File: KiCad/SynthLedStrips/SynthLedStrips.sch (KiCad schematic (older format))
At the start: 38 parts, among them J1 XLR4, J2 XLR4, J3 MIDI IN Kronos DIN-5, J4 MIDI OUT Kronos DIN-5, J5 MIDI IN Acuna DIN-5, J6 MIDI OUT Acuna DIN-5, J7 Conn_01x02_Female, U1 ESP32-WROOM-32, U2 74HC14, U3 74HC14, U4 6N138, U6 6N138

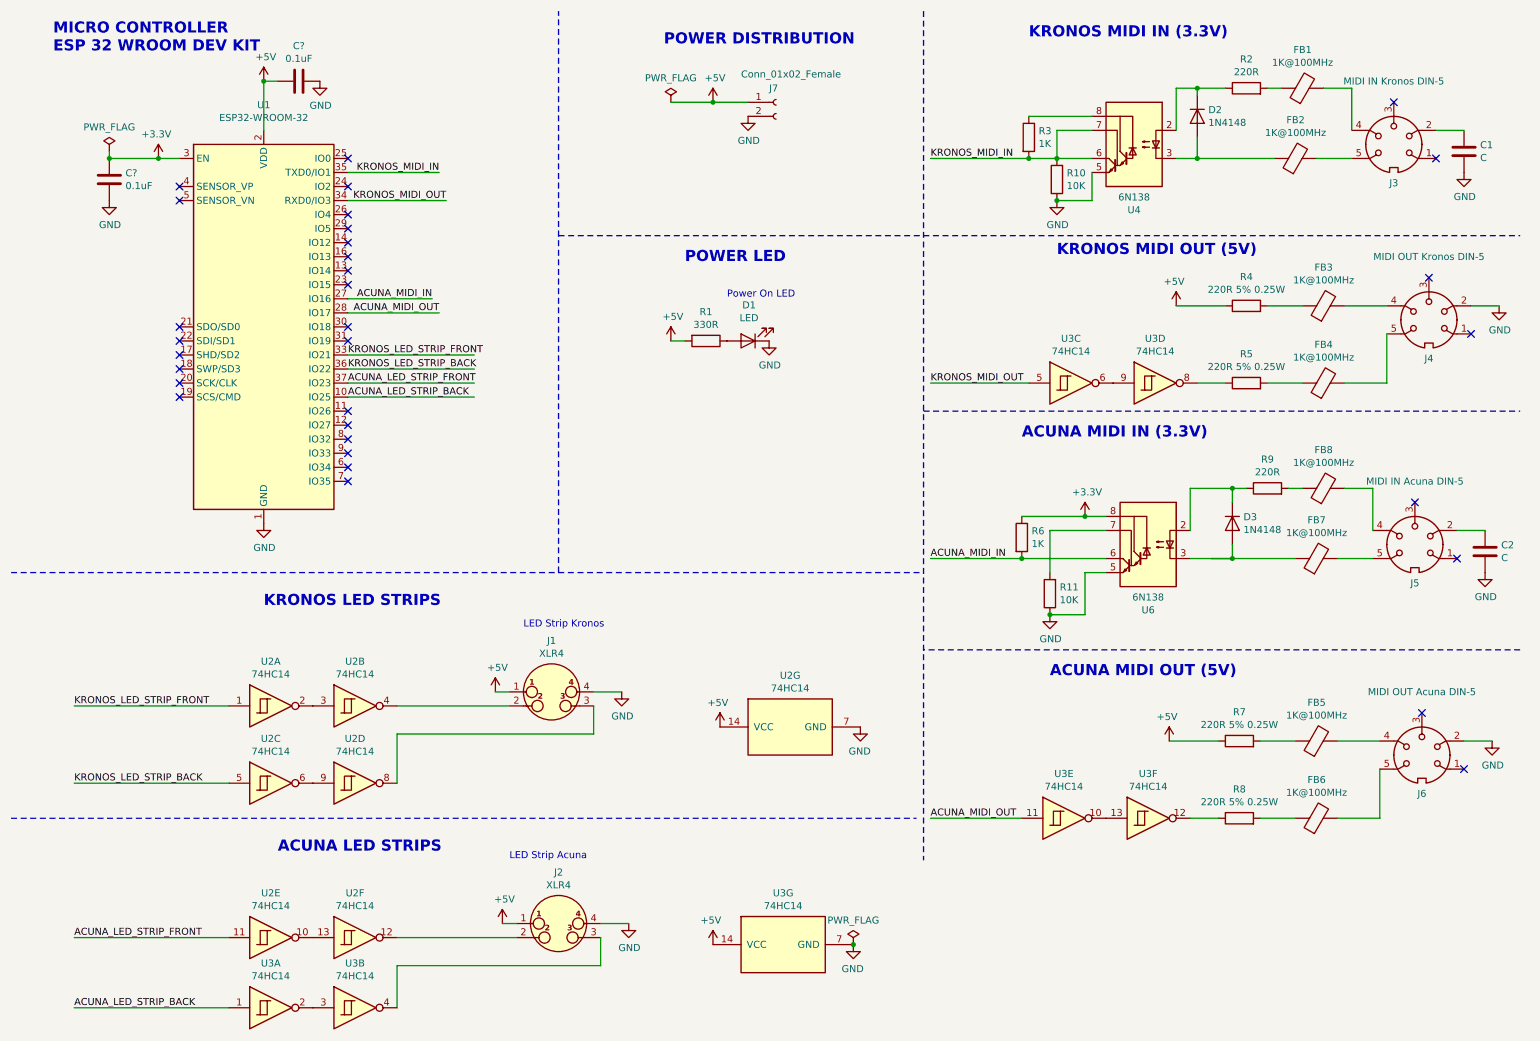
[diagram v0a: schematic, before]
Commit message: KiCad project
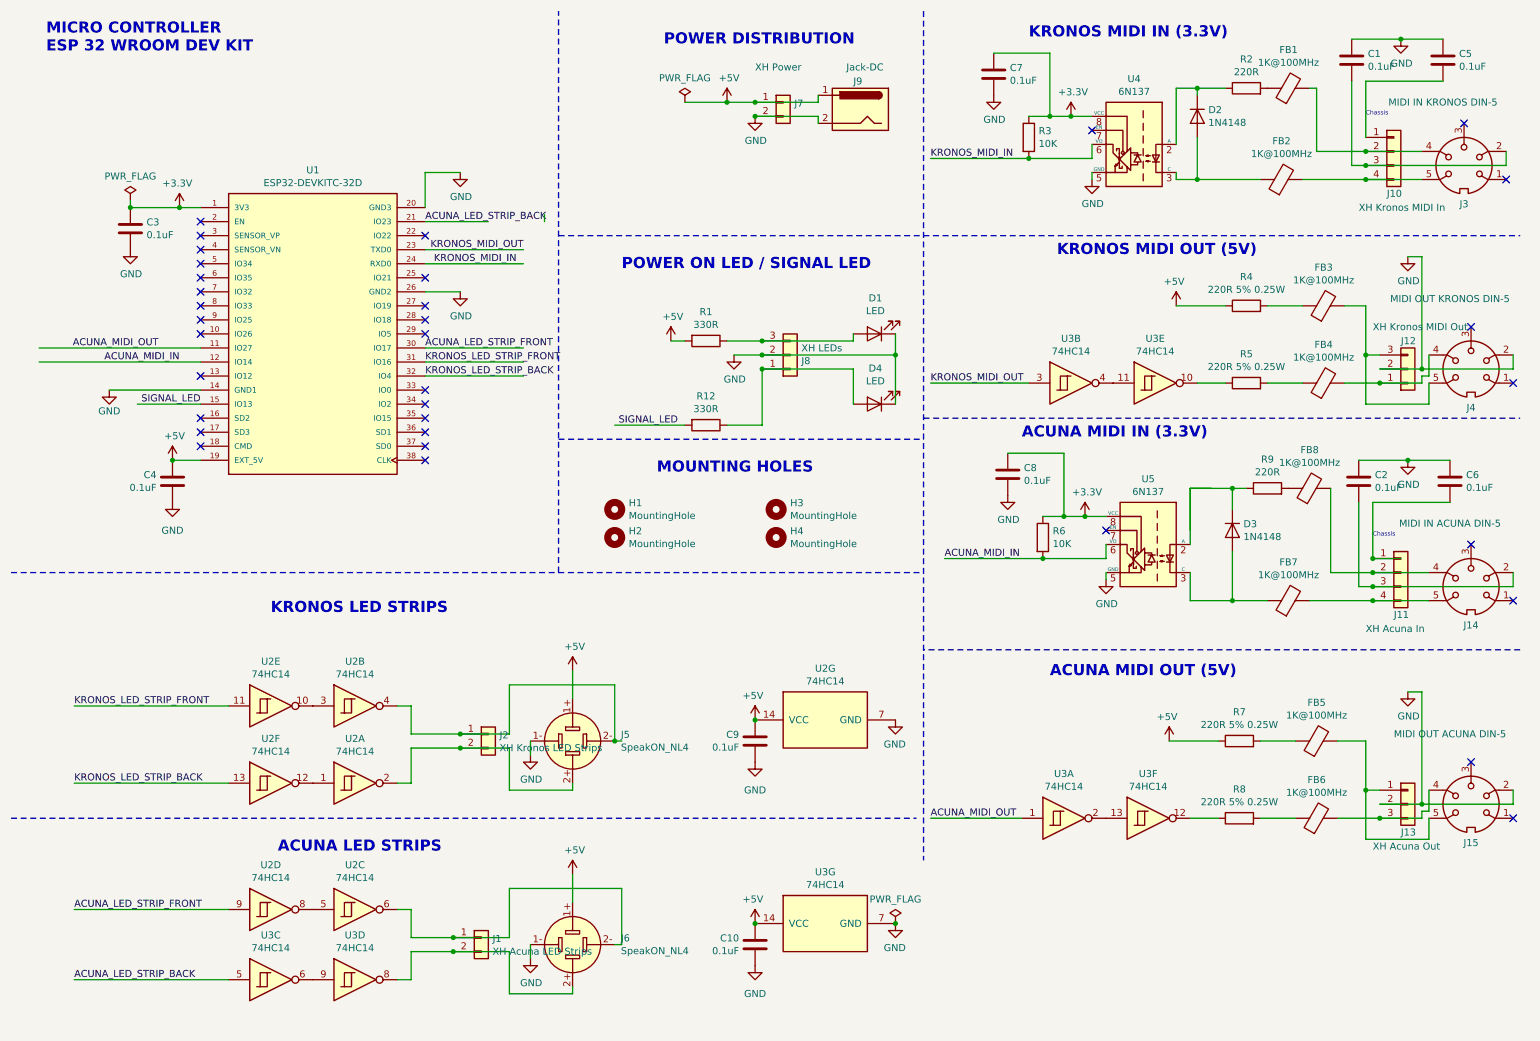
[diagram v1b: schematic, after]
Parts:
- removed J1, J2: XLR4, symbol Connector:XLR4
- removed J5: MIDI IN Acuna DIN-5, symbol Connector:DIN-5
- removed J6: MIDI OUT Acuna DIN-5, symbol Connector:DIN-5
- removed J7: Conn_01x02_Female, symbol Connector:Conn_01x02_Female
- removed R10, R11: 10K, symbol Device:R
- removed U1: ESP32-WROOM-32, RF_Module:ESP32-WROOM-32, symbol RF_Module:ESP32-WROOM-32
- removed U4, U6: 6N138, symbol Isolator:6N138
- added C10, C5, C6, C7, C8, C9: 0.1uF, Capacitor_SMD:C_0805_2012Metric_Pad1.15x1.40mm_HandSolder, symbol Device:C
- added D4: LED, symbol Device:LED
- added H1, H2, H3, H4: MountingHole, MountingHole:MountingHole_4.3mm_M4, symbol Mechanical:MountingHole
- added J1: XH Acuna LED Strips, Connector_JST:JST_XH_B2B-XH-A_1x02_P2.50mm_Vertical, symbol Connector_Generic:Conn_01x02
- added J10: XH Kronos MIDI In, Connector_JST:JST_XH_B4B-XH-A_1x04_P2.50mm_Vertical, symbol Connector_Generic:Conn_01x04
- added J11: XH Acuna In, Connector_JST:JST_XH_B4B-XH-A_1x04_P2.50mm_Vertical, symbol Connector_Generic:Conn_01x04
- added J12: XH Kronos MIDI Out, Connector_JST:JST_XH_B3B-XH-A_1x03_P2.50mm_Vertical, symbol Connector_Generic:Conn_01x03
- added J13: XH Acuna Out, Connector_JST:JST_XH_B3B-XH-A_1x03_P2.50mm_Vertical, symbol Connector_Generic:Conn_01x03
- added J14: MIDI IN ACUNA DIN-5, symbol Connector:DIN-5
- added J15: MIDI OUT ACUNA DIN-5, symbol Connector:DIN-5
- added J2: XH Kronos LED Strips, Connector_JST:JST_XH_B2B-XH-A_1x02_P2.50mm_Vertical, symbol Connector_Generic:Conn_01x02
- added J5, J6: SpeakON_NL4, symbol Connector:SpeakON_NL4
- added J7: XH Power, Connector_JST:JST_XH_B2B-XH-A_1x02_P2.50mm_Vertical, symbol Connector_Generic:Conn_01x02
- added J8: XH LEDs, Connector_JST:JST_XH_B3B-XH-A_1x03_P2.50mm_Vertical, symbol Connector_Generic:Conn_01x03
- added J9: Jack-DC, symbol Connector:Jack-DC
- added R12: 330R, Resistor_SMD:R_0805_2012Metric_Pad1.15x1.40mm_HandSolder, symbol Device:R
- added U1: ESP32-DEVKITC-32D, ESP32_DevKit:MODULE_ESP32-DEVKITC-32D, symbol ESP32_DevKit:ESP32-DEVKITC-32D
- added U4, U5: 6N137, 6N137S:8-SMD, symbol Isolator:6N137
- C1, C2: value C -> 0.1uF; footprint (none) -> Capacitor_SMD:C_0805_2012Metric_Pad1.15x1.40mm_HandSolder
- C3, C4: renamed from C?; footprint (none) -> Capacitor_SMD:C_0805_2012Metric_Pad1.15x1.40mm_HandSolder
- D2, D3: footprint (none) -> Diode_SMD:D_SOD-323_HandSoldering
- FB1, FB2, FB3, FB4, FB5, FB6, FB7, FB8: footprint (none) -> Fuse:Fuse_1210_3225Metric_Pad1.42x2.65mm_HandSolder
- J3: value MIDI IN Kronos DIN-5 -> MIDI IN KRONOS DIN-5
- J4: value MIDI OUT Kronos DIN-5 -> MIDI OUT KRONOS DIN-5
- R1, R2, R9: footprint (none) -> Resistor_SMD:R_0805_2012Metric_Pad1.15x1.40mm_HandSolder
- R3, R6: value 1K -> 10K; footprint (none) -> Resistor_SMD:R_0805_2012Metric_Pad1.15x1.40mm_HandSolder
- R4, R5, R7, R8: footprint (none) -> Resistor_SMD:R_1206_3216Metric_Pad1.42x1.75mm_HandSolder
- U2, U3: footprint (none) -> Package_DIP:DIP-14_W7.62mm
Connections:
- net labels added: SIGNAL_LED
- wire segments 92 -> 181
- no-connect marks 32 -> 34
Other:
- note added: "Chassis"
- note added: "MOUNTING HOLES\n"
- note added: "POWER ON LED / SIGNAL LED\n"
- note removed: "LED Strip Acuna"
- note removed: "LED Strip Kronos"
- note removed: "POWER LED\n"
- note removed: "Power On LED"
- moved on the sheet: C1, C3, C4, D3, FB1, FB2, FB7, FB8, J3, J4, U2A, U2C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
